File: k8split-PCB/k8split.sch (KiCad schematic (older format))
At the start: 242 parts, among them J1 AVR-ISP-6, J13 Breakaway_Tabs, J14 Breakaway_Tabs, J17 Breakaway_Tabs, J18 Breakaway_Tabs, J19 Breakaway_Tabs, J2 AVR-ISP-6, J3 Breakaway_Tabs, J5 Breakaway_Tabs, J6 Breakaway_Tabs, J7 Breakaway_Tabs, J9 Breakaway_Tabs, SW1 SW_Push, SW2 SW_Push, U1 ATmega32U4-AU, U2 ATmega32U4-AU, Y1 16MHz, Y2 16MHz

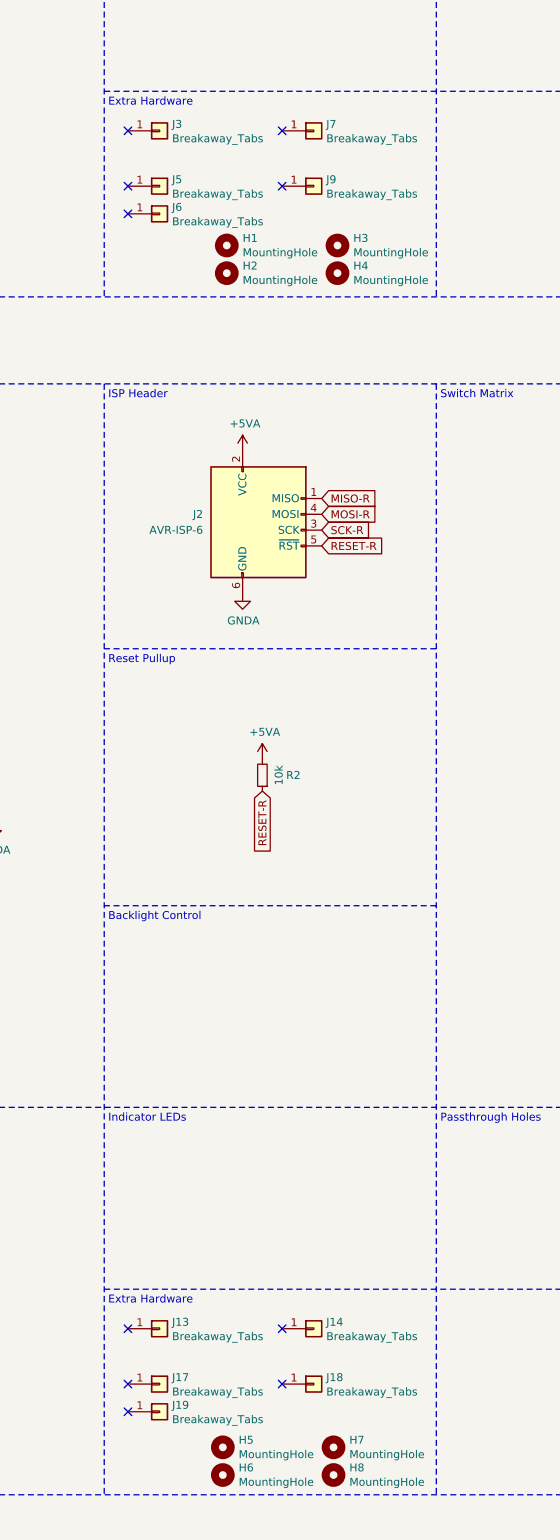
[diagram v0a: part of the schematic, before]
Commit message: initial panelizing
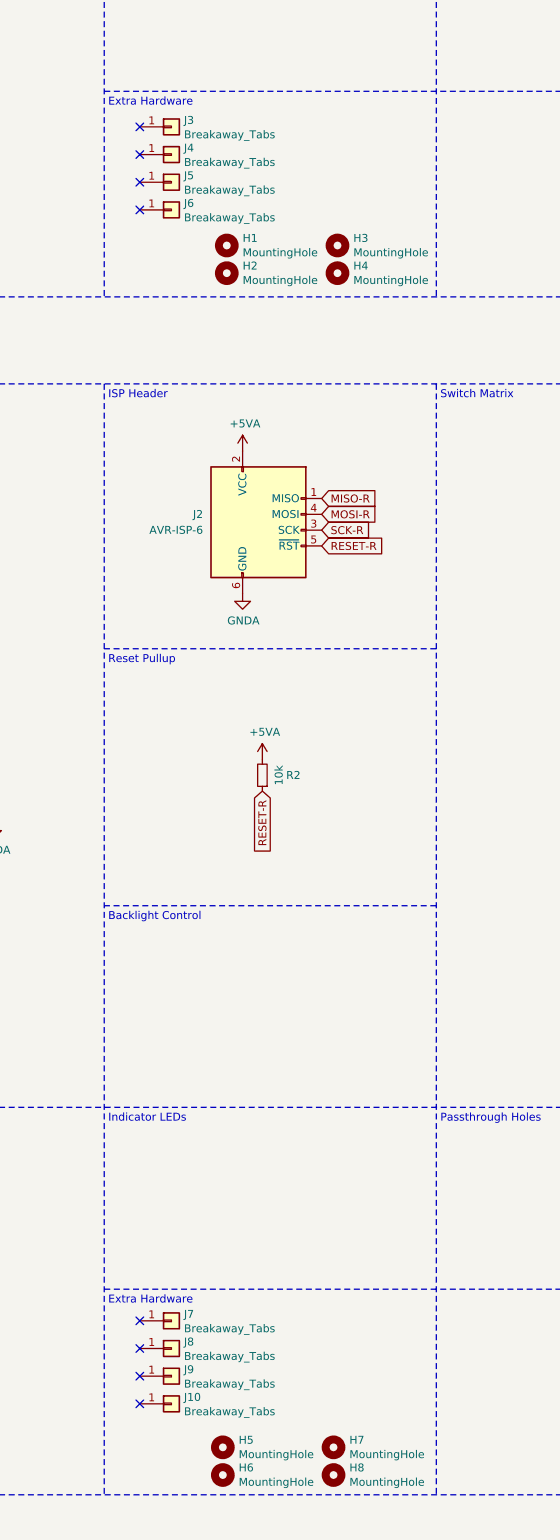
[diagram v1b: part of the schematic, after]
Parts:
- removed J13, J14, J17, J18, J19: Breakaway_Tabs, locallib:breakaway-mousebites, symbol k8split-rescue:Conn_01x01-Connector_Generic-Orbit-rescue
- added J10, J4, J8: Breakaway_Tabs, locallib:breakaway-mousebites, symbol k8split-rescue:Conn_01x01-Connector_Generic-Orbit-rescue
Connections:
- no-connect marks 28 -> 26
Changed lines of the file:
@@
 Text Notes 5675 6500 0    50   ~ 0
 Extra Hardware
-$Comp
-L k8split-rescue:Conn_01x01-Connector_Generic-Orbit-rescue J3
-U 1 1 5BBDC449
-P 6000 6650
-F 0 "J3" H 6079 6692 50  0000 L CNN
-F 1 "Breakaway_Tabs" H 6079 6601 50  0000 L CNN
-F 2 "locallib:breakaway-mousebites" H 6000 6650 50  0001 C CNN
-F 3 "~" H 6000 6650 50  0001 C CNN
-	1    6000 6650
-	1    0    0    -1
-$EndComp
-NoConn ~ 5800 6650
-$Comp
-L k8split-rescue:Conn_01x01-Connector_Generic-Orbit-rescue J5
-U 1 1 5BBF47C0
-P 6000 7000
-F 0 "J5" H 6079 7042 50  0000 L CNN
-F 1 "Breakaway_Tabs" H 6079 6951 50  0000 L CNN
-F 2 "locallib:breakaway-mousebites" H 6000 7000 50  0001 C CNN
-F 3 "~" H 6000 7000 50  0001 C CNN
-	1    6000 7000
-	1    0    0    -1
-$EndComp
-NoConn ~ 5800 7000
-$Comp
-L k8split-rescue:Conn_01x01-Connector_Generic-Orbit-rescue J7
-U 1 1 5BC3C160
-P 6975 6650
-F 0 "J7" H 7054 6692 50  0000 L CNN
-F 1 "Breakaway_Tabs" H 7054 6601 50  0000 L CNN
-F 2 "locallib:breakaway-mousebites" H 6975 6650 50  0001 C CNN
-F 3 "~" H 6975 6650 50  0001 C CNN
-	1    6975 6650
-	1    0    0    -1
-$EndComp
-NoConn ~ 6775 6650
-$Comp
-L k8split-rescue:Conn_01x01-Connector_Generic-Orbit-rescue J9
-U 1 1 5BC3C16F
-P 6975 7000
-F 0 "J9" H 7054 7042 50  0000 L CNN
-F 1 "Breakaway_Tabs" H 7054 6951 50  0000 L CNN
-F 2 "locallib:breakaway-mousebites" H 6975 7000 50  0001 C CNN
-F 3 "~" H 6975 7000 50  0001 C CNN
-	1    6975 7000
-	1    0    0    -1
-$EndComp
-NoConn ~ 6775 7000
 Wire Notes Line
 	7750 11550 5650 11550
@@
 Text Notes 5675 14075 0    50   ~ 0
 Extra Hardware
-$Comp
-L k8split-rescue:Conn_01x01-Connector_Generic-Orbit-rescue J13
-U 1 1 5BCD1D3A
-P 6000 14225
-F 0 "J13" H 6079 14267 50  0000 L CNN
-F 1 "Breakaway_Tabs" H 6079 14176 50  0000 L CNN
-F 2 "locallib:breakaway-mousebites" H 6000 14225 50  0001 C CNN
-F 3 "~" H 6000 14225 50  0001 C CNN
-	1    6000 14225
-	1    0    0    -1
-$EndComp
-NoConn ~ 5800 14225
-$Comp
-L k8split-rescue:Conn_01x01-Connector_Generic-Orbit-rescue J17
-U 1 1 5BCD1D49
-P 6000 14575
-F 0 "J17" H 6079 14617 50  0000 L CNN
-F 1 "Breakaway_Tabs" H 6079 14526 50  0000 L CNN
-F 2 "locallib:breakaway-mousebites" H 6000 14575 50  0001 C CNN
-F 3 "~" H 6000 14575 50  0001 C CNN
-	1    6000 14575
-	1    0    0    -1
-$EndComp
-$Comp
-L k8split-rescue:Conn_01x01-Connector_Generic-Orbit-rescue J19
-U 1 1 5BCD1D50
-P 6000 14750
-F 0 "J19" H 6079 14792 50  0000 L CNN
-F 1 "Breakaway_Tabs" H 6079 14701 50  0000 L CNN
-F 2 "locallib:breakaway-mousebites" H 6000 14750 50  0001 C CNN
-F 3 "~" H 6000 14750 50  0001 C CNN
-	1    6000 14750
-	1    0    0    -1
-$EndComp
-NoConn ~ 5800 14750
-NoConn ~ 5800 14575
-$Comp
-L k8split-rescue:Conn_01x01-Connector_Generic-Orbit-rescue J14
-U 1 1 5BCD1D5A
-P 6975 14225
-F 0 "J14" H 7054 14267 50  0000 L CNN
-F 1 "Breakaway_Tabs" H 7054 14176 50  0000 L CNN
-F 2 "locallib:breakaway-mousebites" H 6975 14225 50  0001 C CNN
-F 3 "~" H 6975 14225 50  0001 C CNN
-	1    6975 14225
-	1    0    0    -1
-$EndComp
-NoConn ~ 6775 14225
-$Comp
-L k8split-rescue:Conn_01x01-Connector_Generic-Orbit-rescue J18
-U 1 1 5BCD1D69
-P 6975 14575
-F 0 "J18" H 7054 14617 50  0000 L CNN
-F 1 "Breakaway_Tabs" H 7054 14526 50  0000 L CNN
-F 2 "locallib:breakaway-mousebites" H 6975 14575 50  0001 C CNN
-F 3 "~" H 6975 14575 50  0001 C CNN
-	1    6975 14575
-	1    0    0    -1
-$EndComp
-NoConn ~ 6775 14575
 Text Notes 13050 7650 0    50   ~ 10
 LEFT HAND SCHEMATIC
@@
 Wire Notes Line
 	5650 675  5650 7700
-NoConn ~ 5800 7175
-$Comp
-L k8split-rescue:Conn_01x01-Connector_Generic-Orbit-rescue J6
-U 1 1 5BBF48DE
-P 6000 7175
-F 0 "J6" H 6079 7217 50  0000 L CNN
-F 1 "Breakaway_Tabs" H 6079 7126 50  0000 L CNN
-F 2 "locallib:breakaway-mousebites" H 6000 7175 50  0001 C CNN
-F 3 "~" H 6000 7175 50  0001 C CNN
-	1    6000 7175
-	1    0    0    -1
-$EndComp
 Connection ~ 1100 11550
 Connection ~ 1100 11350
@@
 	1575 3875 2425 3875
 $Comp
-L Mechanical:MountingHole H1
-U 1 1 5E3013F1
-P 6425 7375
-F 0 "H1" H 6525 7421 50  0000 L CNN
-F 1 "MountingHole" H 6525 7330 50  0000 L CNN
-F 2 "MountingHole:MountingHole_3.2mm_M3" H 6425 7375 50  0001 C CNN
-F 3 "~" H 6425 7375 50  0001 C CNN
-	1    6425 7375
-	1    0    0    -1
-$EndComp
-$Comp
 L Mechanical:MountingHole H2
 U 1 1 5E3013F7
@@
 	1    0    0    -1
 $EndComp
+$Comp
+L k8split-rescue:Conn_01x01-Connector_Generic-Orbit-rescue J3
+U 1 1 5E2DC692
+P 6075 6625
+F 0 "J3" H 6154 6667 50  0000 L CNN
+F 1 "Breakaway_Tabs" H 6154 6576 50  0000 L CNN
+F 2 "locallib:breakaway-mousebites" H 6075 6625 50  0001 C CNN
+F 3 "~" H 6075 6625 50  0001 C CNN
+	1    6075 6625
+	1    0    0    -1
+$EndComp
+NoConn ~ 5875 6625
+NoConn ~ 5875 6800
+$Comp
+L k8split-rescue:Conn_01x01-Connector_Generic-Orbit-rescue J6
+U 1 1 5E2DC6A0
+P 6075 7150
+F 0 "J6" H 6154 7192 50  0000 L CNN
+F 1 "Breakaway_Tabs" H 6154 7101 50  0000 L CNN
+F 2 "locallib:breakaway-mousebites" H 6075 7150 50  0001 C CNN
+F 3 "~" H 6075 7150 50  0001 C CNN
+	1    6075 7150
+	1    0    0    -1
+$EndComp
+NoConn ~ 5875 7150
+$Comp
+L k8split-rescue:Conn_01x01-Connector_Generic-Orbit-rescue J4
+U 1 1 5E2DC699
+P 6075 6800
+F 0 "J4" H 6154 6842 50  0000 L CNN
+F 1 "Breakaway_Tabs" H 6154 6751 50  0000 L CNN
+F 2 "locallib:breakaway-mousebites" H 6075 6800 50  0001 C CNN
+F 3 "~" H 6075 6800 50  0001 C CNN
+	1    6075 6800
+	1    0    0    -1
+$EndComp
+$Comp
+L k8split-rescue:Conn_01x01-Connector_Generic-Orbit-rescue J5
+U 1 1 5E2DC6AF
+P 6075 6975
+F 0 "J5" H 6154 7017 50  0000 L CNN
+F 1 "Breakaway_Tabs" H 6154 6926 50  0000 L CNN
+F 2 "locallib:breakaway-mousebites" H 6075 6975 50  0001 C CNN
+F 3 "~" H 6075 6975 50  0001 C CNN
+	1    6075 6975
+	1    0    0    -1
+$EndComp
+NoConn ~ 5875 6975
+$Comp
+L Mechanical:MountingHole H1
+U 1 1 5E3013F1
+P 6425 7375
+F 0 "H1" H 6525 7421 50  0000 L CNN
+F 1 "MountingHole" H 6525 7330 50  0000 L CNN
+F 2 "MountingHole:MountingHole_3.2mm_M3" H 6425 7375 50  0001 C CNN
+F 3 "~" H 6425 7375 50  0001 C CNN
+	1    6425 7375
+	1    0    0    -1
+$EndComp
+$Comp
+L k8split-rescue:Conn_01x01-Connector_Generic-Orbit-rescue J7
+U 1 1 5E3F5C7F
+P 6075 14175
+F 0 "J7" H 6154 14217 50  0000 L CNN
+F 1 "Breakaway_Tabs" H 6154 14126 50  0000 L CNN
+F 2 "locallib:breakaway-mousebites" H 6075 14175 50  0001 C CNN
+F 3 "~" H 6075 14175 50  0001 C CNN
+	1    6075 14175
+	1    0    0    -1
+$EndComp
+NoConn ~ 5875 14175
+NoConn ~ 5875 14350
+$Comp
+L k8split-rescue:Conn_01x01-Connector_Generic-Orbit-rescue J10
+U 1 1 5E3F5C87
+P 6075 14700
+F 0 "J10" H 6154 14742 50  0000 L CNN
+F 1 "Breakaway_Tabs" H 6154 14651 50  0000 L CNN
+F 2 "locallib:breakaway-mousebites" H 6075 14700 50  0001 C CNN
+F 3 "~" H 6075 14700 50  0001 C CNN
+	1    6075 14700
+	1    0    0    -1
+$EndComp
+NoConn ~ 5875 14700
+$Comp
+L k8split-rescue:Conn_01x01-Connector_Generic-Orbit-rescue J8
+U 1 1 5E3F5C8E
+P 6075 14350
+F 0 "J8" H 6154 14392 50  0000 L CNN
+F 1 "Breakaway_Tabs" H 6154 14301 50  0000 L CNN
+F 2 "locallib:breakaway-mousebites" H 6075 14350 50  0001 C CNN
+F 3 "~" H 6075 14350 50  0001 C CNN
+	1    6075 14350
+	1    0    0    -1
+$EndComp
+$Comp
+L k8split-rescue:Conn_01x01-Connector_Generic-Orbit-rescue J9
+U 1 1 5E3F5C94
+P 6075 14525
+F 0 "J9" H 6154 14567 50  0000 L CNN
+F 1 "Breakaway_Tabs" H 6154 14476 50  0000 L CNN
+F 2 "locallib:breakaway-mousebites" H 6075 14525 50  0001 C CNN
+F 3 "~" H 6075 14525 50  0001 C CNN
+	1    6075 14525
+	1    0    0    -1
+$EndComp
+NoConn ~ 5875 14525
 $EndSCHEMATC
